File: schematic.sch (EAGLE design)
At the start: 5 parts, among them P1 TYPE-C-16PIN, U1 ME6211C33M5G

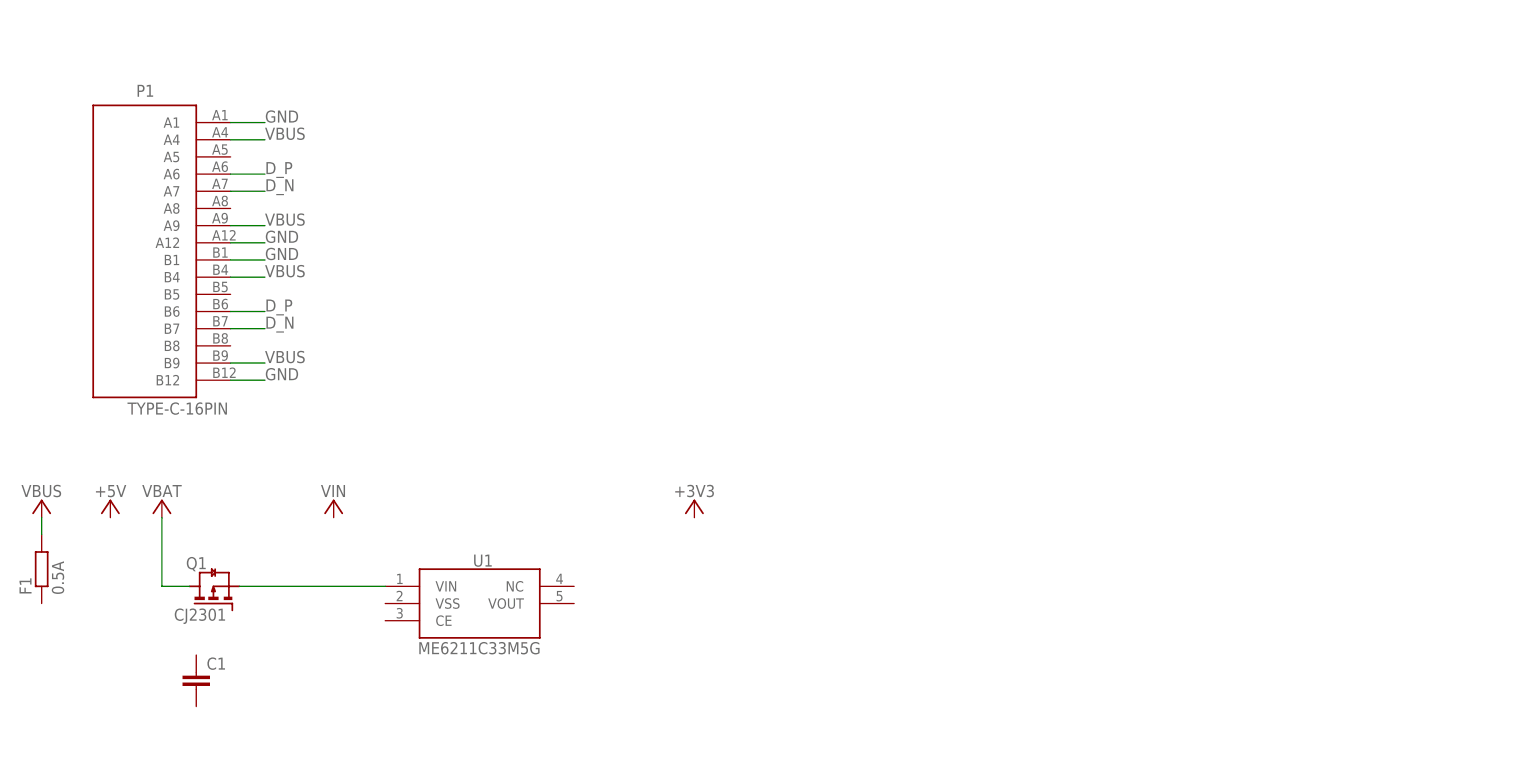
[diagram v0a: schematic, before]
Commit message: .
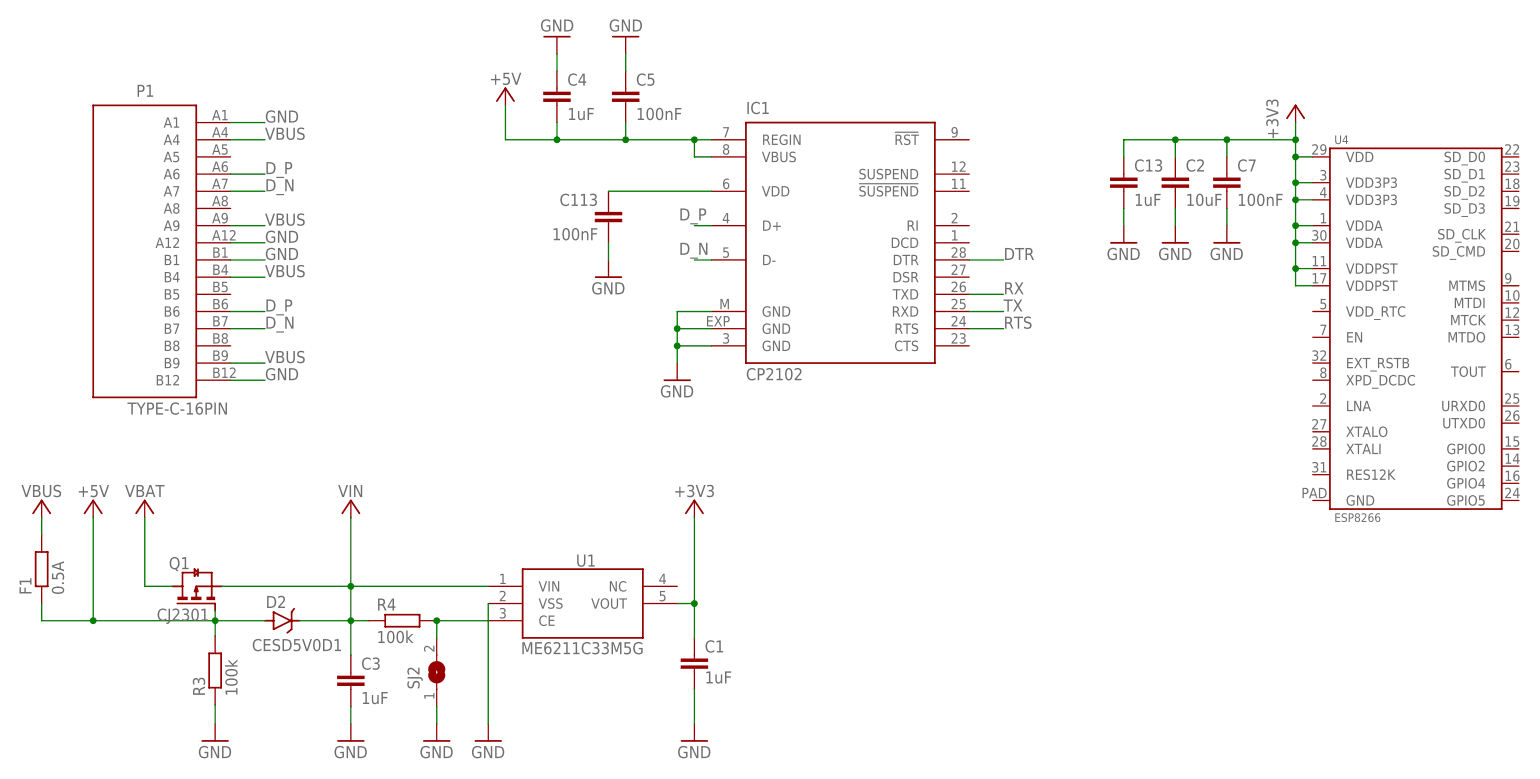
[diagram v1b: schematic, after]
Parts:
- added C113, C5, C7: 100nF, rcl:C-EUC0402
- added C13, C3, C4: 1uF, rcl:C-EUC0402
- added C2: 10uF, rcl:C-EUC0402
- added D2: CESD5V0D1, Diodes:CESD5V0D1
- added IC1: CP2102, silabs:CP2102
- added R3, R4: 100k, rcl:R-EU_R0402
- added SJ2: (no value), jumper:SJ
- added U4: ESP8266, Espressif:ESP8266
- C1: value (none) -> 1uF
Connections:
- removed net N$2: Q1.2, U1.VIN
- new net +3V3: C13.1, C2.1, C7.1, U4.VDD, U4.VDD3P3@1, U4.VDD3P3@2, U4.VDDA@1, U4.VDDA@2, U4.VDDPST@1, U4.VDDPST@2
- new net +5V: D2.A, F1.1, Q1.1, R3.2
- new net DTR: IC1.DTR
- new net EN: R4.2, SJ2.2, U1.CE
- new net N$1: C113.1, IC1.VDD
- new net POWER: C4.2, C5.2, IC1.REGIN, IC1.VBUS
- new net RTS: IC1.RTS
- new net RX: IC1.TXD
- new net TX: IC1.RXD
- new net VIN: C1.1, C3.1, D2.C, Q1.2, R4.1, U1.VIN, U1.VOUT
- net D_N: now also IC1.D-
- net D_P: now also IC1.D+
- net GND: now also C1.2, C113.2, C13.2, C2.2, C3.2, C4.1, C5.1, C7.2, IC1.GND, IC1.GND@EXP, IC1.GND@M, R3.1, SJ2.1, U1.VSS
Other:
- moved on the sheet: C1, Q1, U1
